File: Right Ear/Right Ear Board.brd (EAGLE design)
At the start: 39.4 x 20.3 mm, 8 parts, among them J1 502585-0470

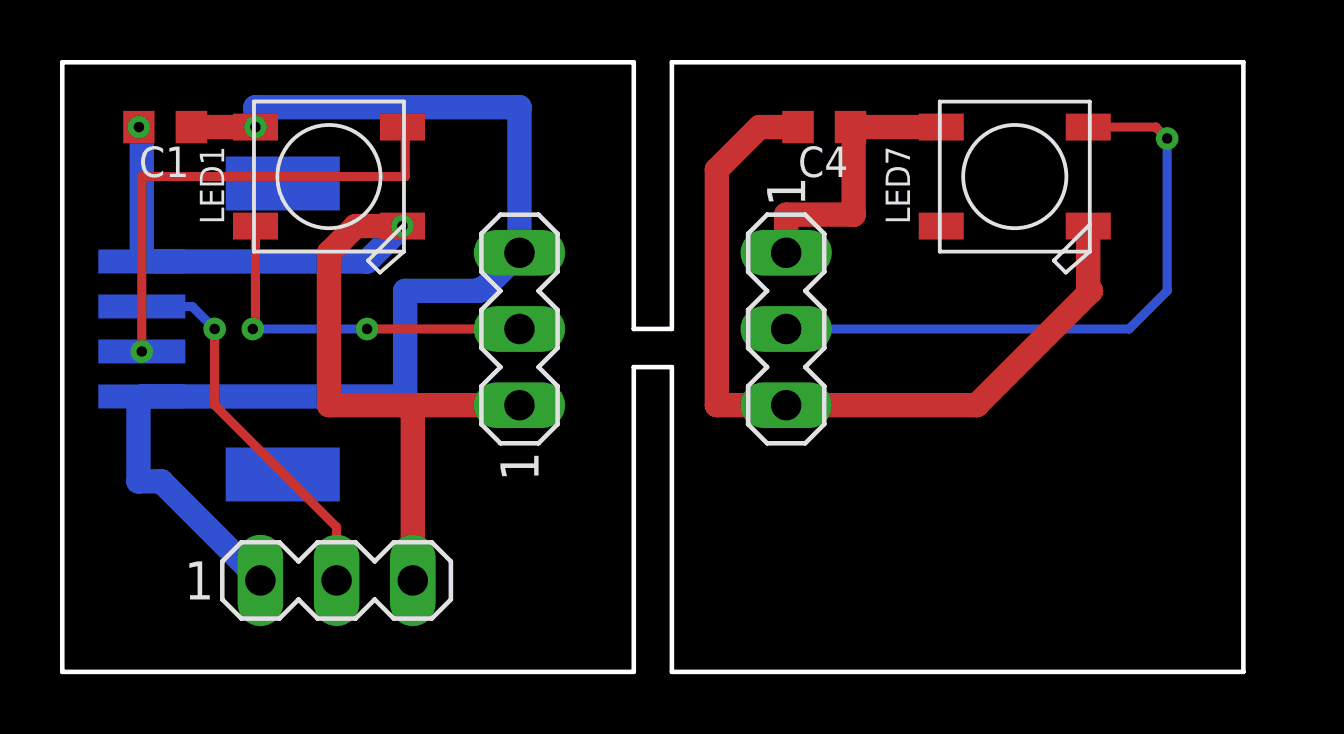
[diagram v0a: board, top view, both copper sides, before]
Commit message: Redid right ear board layouts
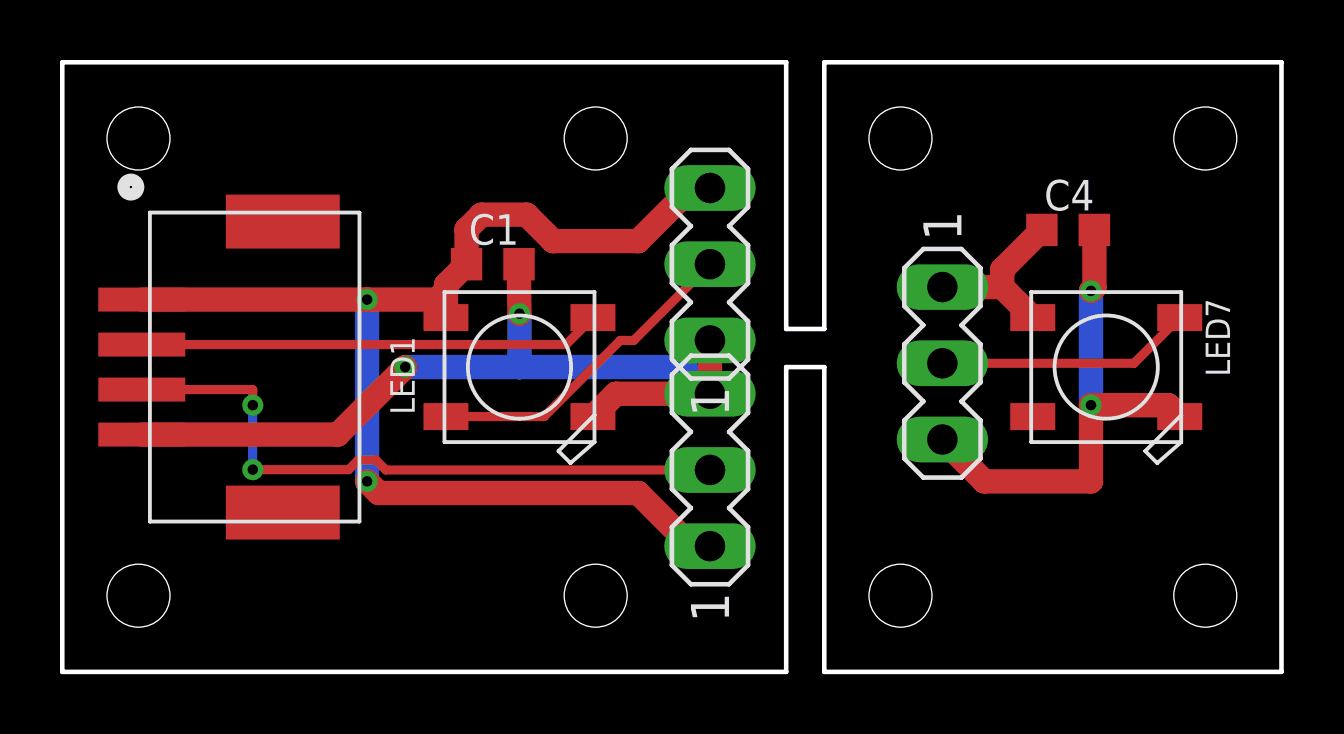
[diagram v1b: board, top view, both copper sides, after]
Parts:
- moved SV1 13.0 mm to (21.6, 6.73), turned to 90 degrees
- moved C1 11.8 mm to (14.4, 13.6), turned to 0 degrees
- moved LED1 8.98 mm to (15.2, 10.2)
- moved C4 8.82 mm to (33.5, 14.7), turned to 0 degrees
- moved LED7 7.04 mm to (34.8, 10.2)
- moved SV3 6.71 mm to (21.6, 13.6)
- moved SV2 5.33 mm to (29.3, 10.3)
- moved J1 1.27 mm to (6.35, 10.2), flipped to the top, turned to 90 degrees
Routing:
- net GND: track 61.3 -> 46.7 mm, vias 2 -> 4
- net DATA: track 33.5 -> 19.4 mm, vias 3 -> 0
- net SERVO_PWM: track 12.8 -> 21.9 mm, vias 1 -> 2
- net +5V: track 50.9 -> 47.3 mm, vias 1 -> 2
- net DI: track 16.3 -> 15.4 mm, vias 1 -> 0
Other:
- board size 39.4 x 20.3 mm -> 40.6 x 20.3 mm
